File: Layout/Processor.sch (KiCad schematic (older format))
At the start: 9 parts, among them J5 Conn_01x02_Female, J6 Conn_01x02_Female, SW1 SW_Push, U1 DSPIC33FJ128MC804

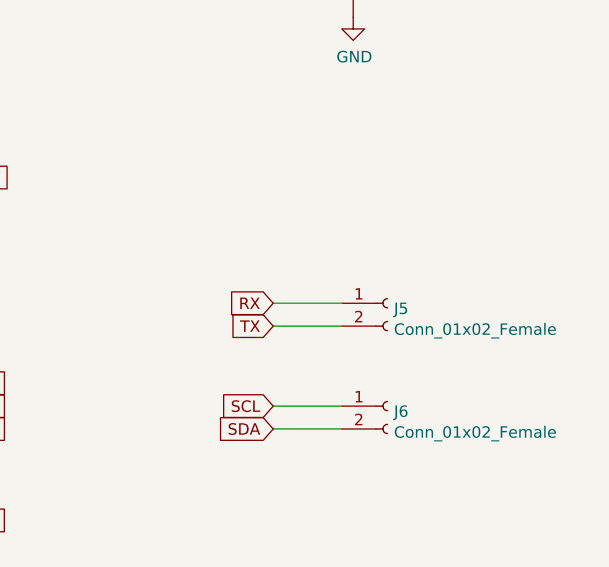
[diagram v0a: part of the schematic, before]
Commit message: Layout
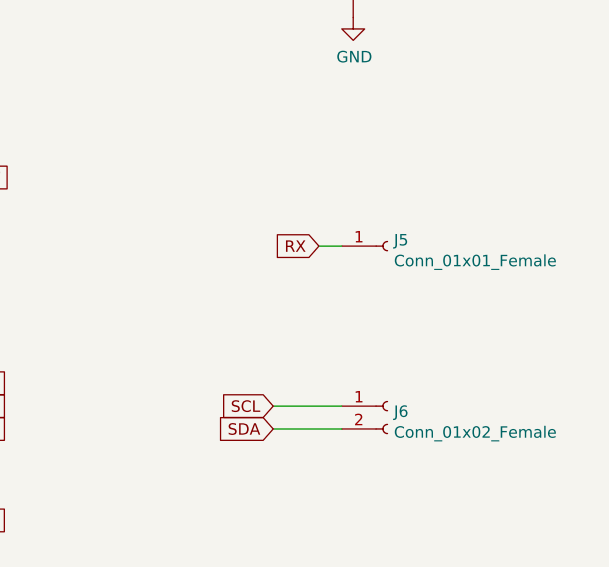
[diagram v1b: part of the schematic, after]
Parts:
- removed J5: Conn_01x02_Female, Connector_PinSocket_2.54mm:PinSocket_1x02_P2.54mm_Vertical, symbol Connector:Conn_01x02_Female
- added J5: Conn_01x01_Female, Connector_PinSocket_2.54mm:PinSocket_1x01_P2.54mm_Vertical, symbol Connector:Conn_01x01_Female
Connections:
- net RX: now also J5.1 (Pin_1)
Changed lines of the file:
@@
 	5600 5500 5600 5400
-$Comp
-L Connector:Conn_01x02_Female J5
-U 1 1 5F5B5019
-P 9650 2750
-F 0 "J5" H 9678 2726 50  0000 L CNN
-F 1 "Conn_01x02_Female" H 9678 2635 50  0000 L CNN
-F 2 "Connector_PinSocket_2.54mm:PinSocket_1x02_P2.54mm_Vertical" H 9650 2750 50  0001 C CNN
-F 3 "~" H 9650 2750 50  0001 C CNN
-	1    9650 2750
-	1    0    0    -1
-$EndComp
 $Comp
 L Connector:Conn_01x02_Female J6
@@
 $EndComp
 Wire Wire Line
-	9450 2750 9150 2750
-Wire Wire Line
-	9450 2850 9150 2850
-Wire Wire Line
 	9450 3200 9150 3200
 Wire Wire Line
 	9450 3300 9150 3300
-Text GLabel 9150 2750 0    50   Input ~ 0
+Text GLabel 9350 2500 0    50   Input ~ 0
 RX
-Text GLabel 9150 2850 0    50   Input ~ 0
-TX
 Text GLabel 9150 3200 0    50   Input ~ 0
 SCL
 Text GLabel 9150 3300 0    50   Input ~ 0
 SDA
+$Comp
+L Connector:Conn_01x01_Female J5
+U 1 1 5F729F19
+P 9650 2500
+F 0 "J5" H 9678 2526 50  0000 L CNN
+F 1 "Conn_01x01_Female" H 9678 2435 50  0000 L CNN
+F 2 "Connector_PinSocket_2.54mm:PinSocket_1x01_P2.54mm_Vertical" H 9650 2500 50  0001 C CNN
+F 3 "~" H 9650 2500 50  0001 C CNN
+	1    9650 2500
+	1    0    0    -1
+$EndComp
+Wire Wire Line
+	9350 2500 9450 2500
 $EndSCHEMATC
